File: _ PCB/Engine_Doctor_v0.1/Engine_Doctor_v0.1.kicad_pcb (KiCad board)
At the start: 2 copper layers, 1 part, among them U1 lolin32_lite_V1.00

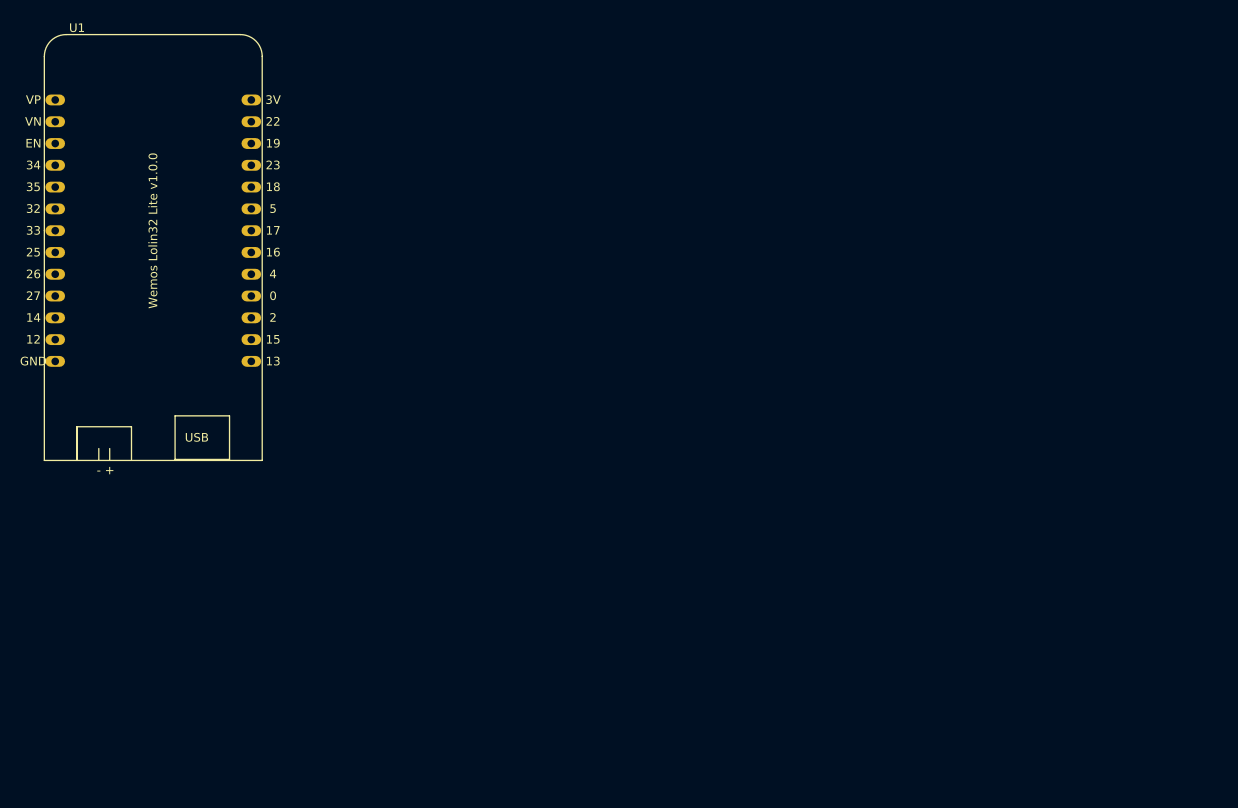
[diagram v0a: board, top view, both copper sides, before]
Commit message: V0.1 PCB Design Complete
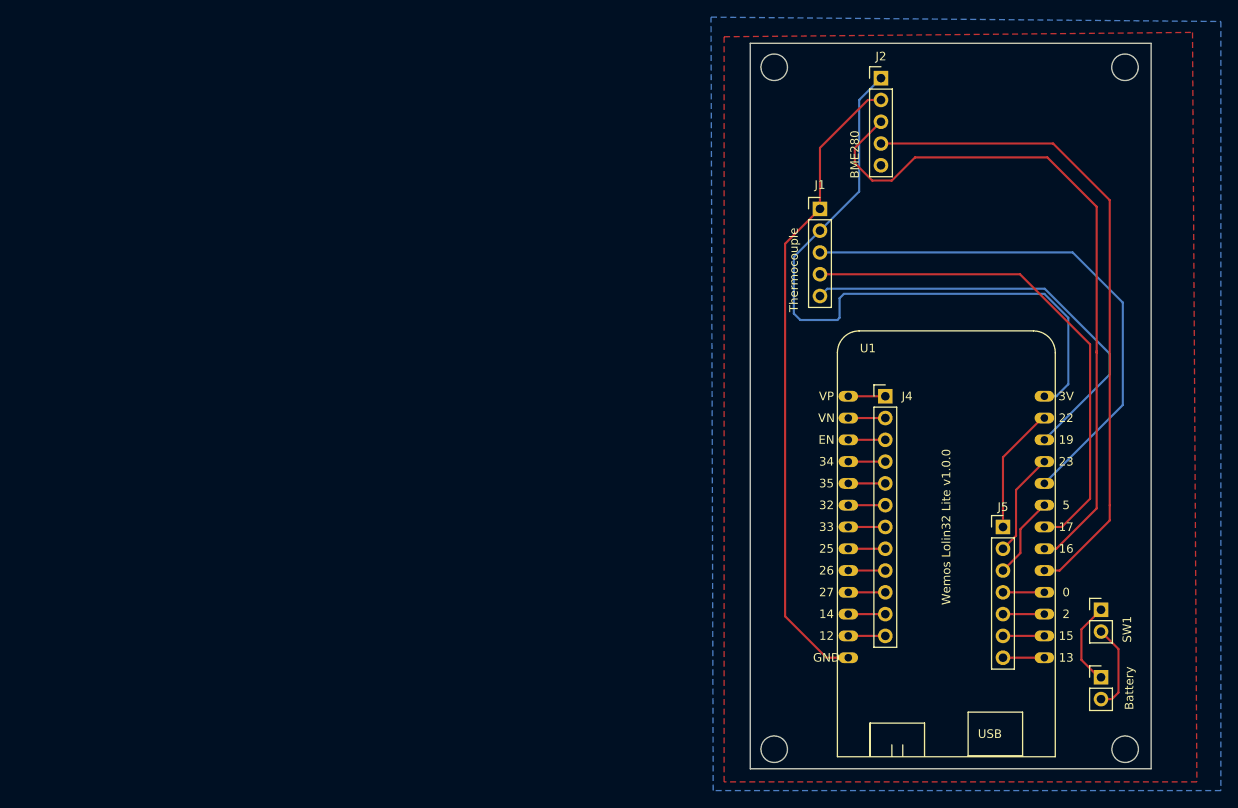
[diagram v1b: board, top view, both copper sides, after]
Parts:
- added J1: Thermocouple, Connector_PinHeader_2.54mm:PinHeader_1x05_P2.54mm_Vertical, F.Cu at (186.2, 95.5)
- added J2: BME280, Connector_PinHeader_2.54mm:PinHeader_1x05_P2.54mm_Vertical, F.Cu at (193.3, 80.3)
- added J3: Battery, Connector_PinHeader_2.54mm:PinHeader_1x02_P2.54mm_Vertical, F.Cu at (218.9, 150.1)
- added J4: Spare2, Connector_PinHeader_2.54mm:PinHeader_1x12_P2.54mm_Vertical, F.Cu at (193.8, 117.3)
- added J5: Spare1, Connector_PinHeader_2.54mm:PinHeader_1x07_P2.54mm_Vertical, F.Cu at (207.5, 132.6)
- added REF**: OSHW-Logo2_7.3x6mm_SilkScreen, Symbol:OSHW-Logo2_7.3x6mm_SilkScreen, B.Cu at (205.7, 119.1)
- added SW1: Power Switch, Connector_PinHeader_2.54mm:PinHeader_1x02_P2.54mm_Vertical, F.Cu at (218.9, 142.2)
- moved U1 98.7 mm to (200.9, 132.6)
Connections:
- U1 pad 1: Net-(U1-Pad1) -> SVP
- U1 pad 10: Net-(U1-Pad10) -> S27
- U1 pad 11: Net-(U1-Pad11) -> S14
- U1 pad 12: Net-(U1-Pad12) -> S12
- U1 pad 13: Net-(U1-Pad13) -> GND
- U1 pad 14: Net-(U1-Pad14) -> S13
- U1 pad 15: Net-(U1-Pad15) -> S15
- U1 pad 16: Net-(U1-Pad16) -> S2
- U1 pad 17: Net-(U1-Pad17) -> S0
- U1 pad 18: Net-(U1-Pad18) -> SDA
- U1 pad 19: Net-(U1-Pad19) -> SCL
- U1 pad 2: Net-(U1-Pad2) -> SVN
- U1 pad 20: Net-(U1-Pad20) -> CS
- U1 pad 21: Net-(U1-Pad21) -> S5
- U1 pad 22: Net-(U1-Pad22) -> SCK
- U1 pad 23: Net-(U1-Pad23) -> S23
- U1 pad 24: Net-(U1-Pad24) -> SO
- U1 pad 25: Net-(U1-Pad25) -> S22
- U1 pad 26: Net-(U1-Pad26) -> 3v3
- U1 pad 3: Net-(U1-Pad3) -> SEN
- U1 pad 4: Net-(U1-Pad4) -> S34
- U1 pad 5: Net-(U1-Pad5) -> S35
- U1 pad 6: Net-(U1-Pad6) -> S32
- U1 pad 7: Net-(U1-Pad7) -> S33
- U1 pad 8: Net-(U1-Pad8) -> S25
- U1 pad 9: Net-(U1-Pad9) -> S26
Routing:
- net SCL: track 0.00 -> 82.0 mm
- net 3v3: track 0.00 -> 78.8 mm
- net SDA: track 0.00 -> 76.8 mm
- net GND: track 0.00 -> 75.1 mm
- net SCK: track 0.00 -> 62.6 mm
- net CS: track 0.00 -> 59.6 mm
- net SO: track 0.00 -> 50.5 mm
- net S22: track 0.00 -> 14.8 mm
- net S23: track 0.00 -> 12.2 mm
- net Net-(J3-Pad2): track 0.00 -> 10.3 mm
- net Net-(J3-Pad1): track 0.00 -> 9.92 mm
- net S5: track 0.00 -> 9.62 mm
- net S2: track 0.00 -> 4.83 mm
- net S15: track 0.00 -> 4.83 mm
- net S13: track 0.00 -> 4.83 mm
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- added copper zone on B.Cu, net GND
- added copper zone on F.Cu, net GND
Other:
- board outline added: 46.7 x 84.6 mm
- board text added: "ENGINE DOCTOR V0.1 WWW.MKME.ORG"
